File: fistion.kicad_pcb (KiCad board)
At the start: 2 copper layers, 165 x 92.1 mm, 67 parts, among them J1 Conn_01x07, J2 Conn_01x07, J3 Conn_01x04, U1 nice_nano, U2 MT25QL128ABA1ESE

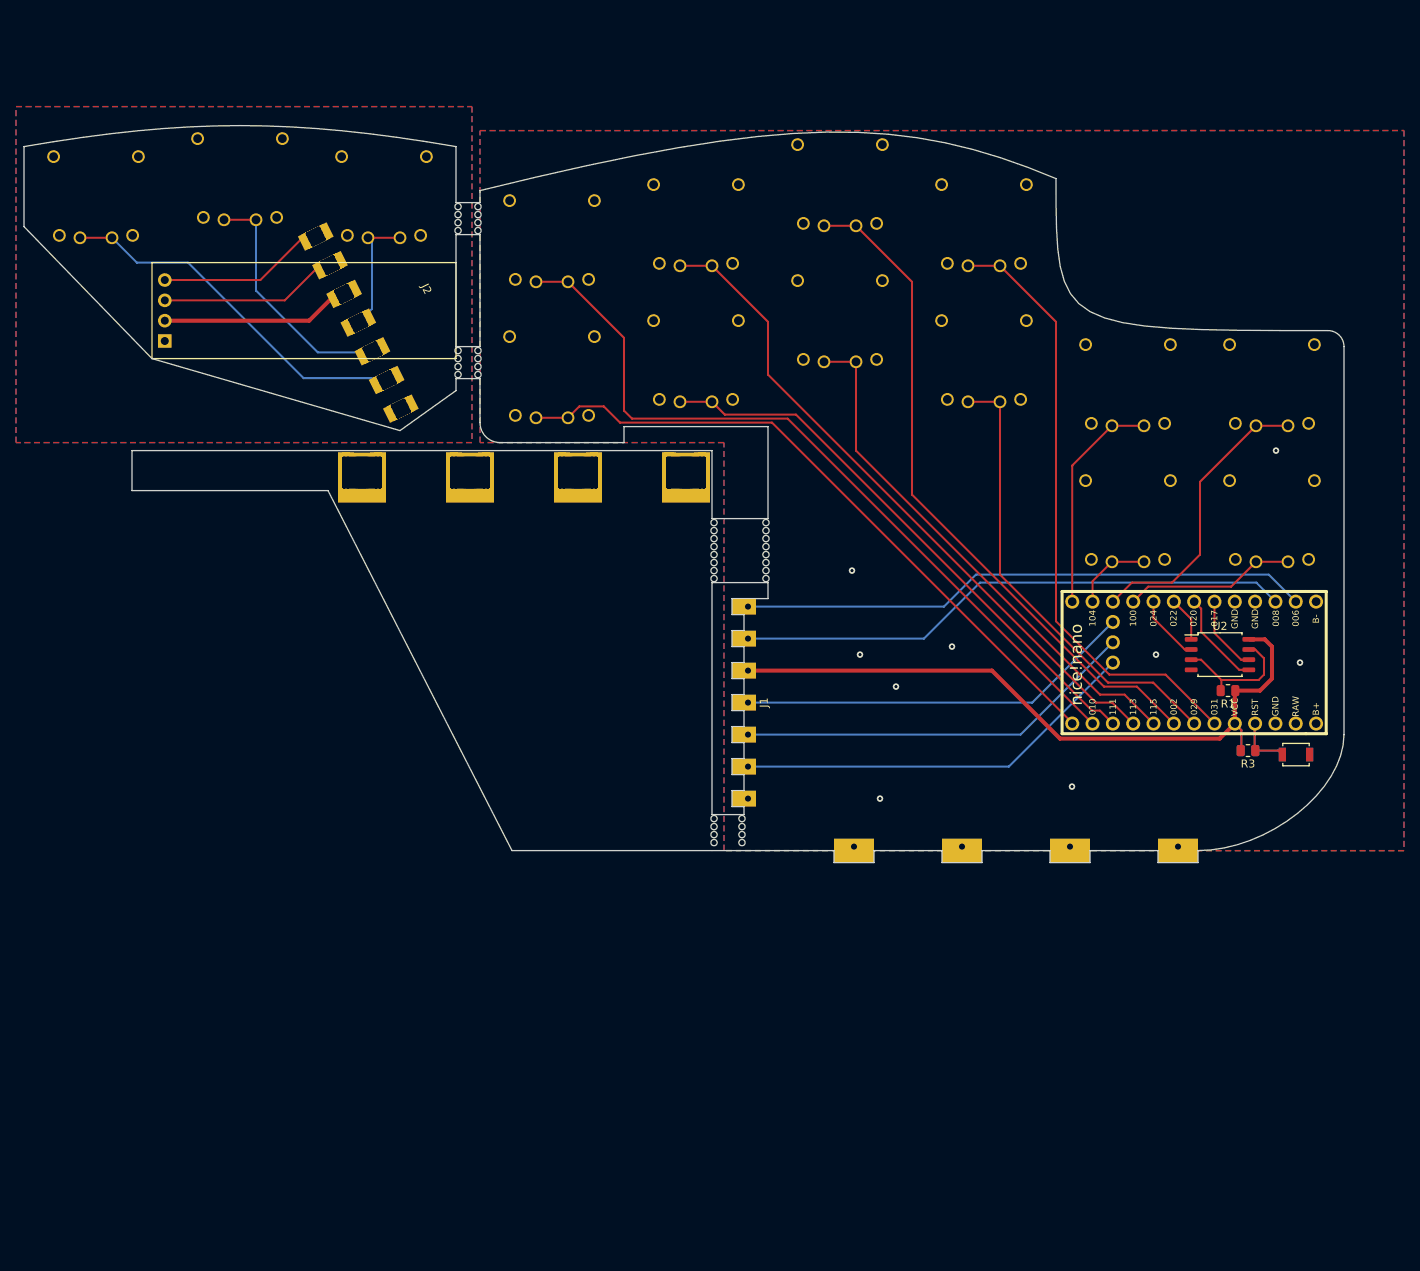
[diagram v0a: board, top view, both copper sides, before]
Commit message: Pending
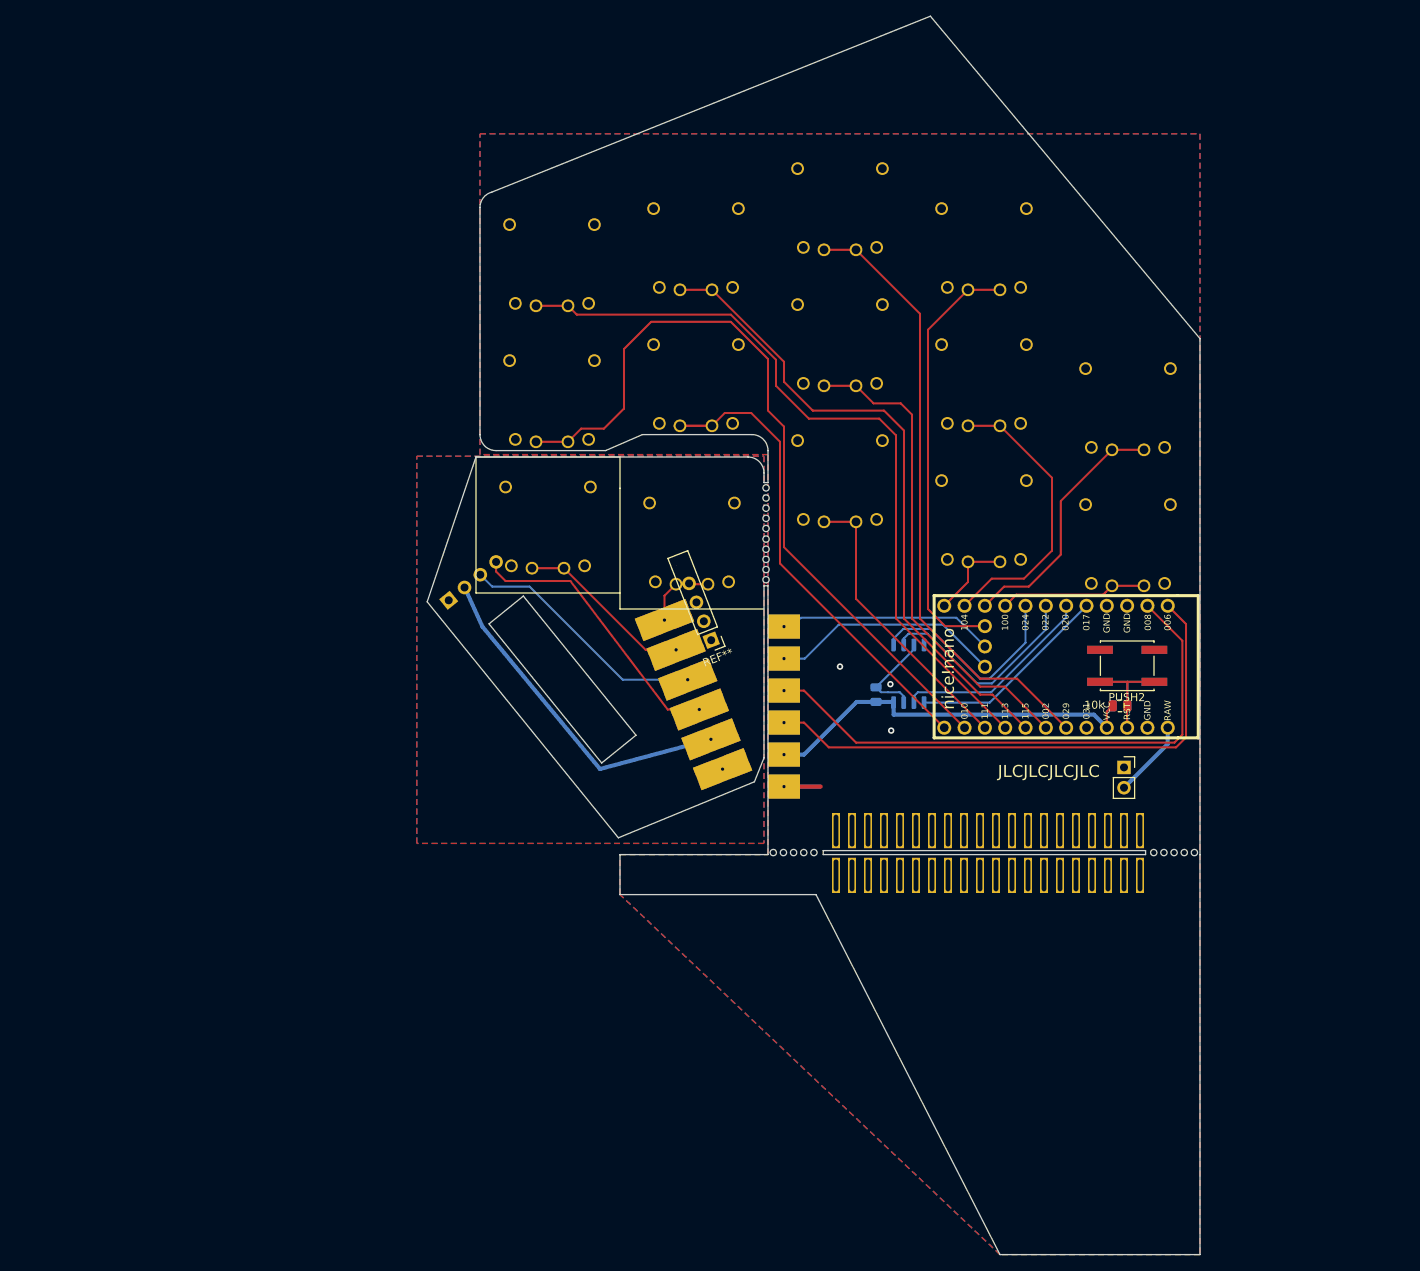
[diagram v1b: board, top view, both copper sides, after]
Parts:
- removed KEY15: SW_Push, lib:Kailh_PG1232
- removed the KEY6 at (169.0, 52.0)
- removed the REF** at (106.0, 71.5)
- removed the REF** at (99.0, 75.5)
- removed the REF** at (99.0, 73.5)
- removed the REF** at (99.0, 76.5)
- removed the REF** at (99.0, 70.5)
- removed the REF** at (99.0, 71.5)
- removed the REF** at (99.0, 69.5)
- removed the REF** at (99.0, 72.5)
- removed the REF** at (103.0, 108.5)
- removed the REF** at (103.0, 107.5)
- removed the REF** at (103.0, 109.5)
- removed the REF** at (106.0, 70.5)
- removed the REF** at (103.0, 106.5)
- removed the REF** at (99.0, 107.5)
- removed the REF** at (99.0, 108.5)
- removed the REF** at (99.0, 106.5)
- removed the REF** at (99.0, 109.5)
- removed the REF** at (70.0, 32.0)
- removed the REF** at (70.0, 31.0)
- removed the REF** at (70.0, 33.0)
- removed the REF** at (70.0, 30.0)
- removed the REF** at (67.0, 31.0)
- removed the REF** at (106.0, 72.5)
- removed the REF** at (67.0, 32.0)
- removed the REF** at (67.0, 30.0)
- removed the REF** at (67.0, 33.0)
- removed the REF** at (70.0, 50.0)
- removed the REF** at (70.0, 49.0)
- removed the REF** at (70.0, 51.0)
- removed the REF** at (70.0, 48.0)
- removed the REF** at (67.0, 49.0)
- removed the REF** at (67.0, 50.0)
- removed the REF** at (67.0, 48.0)
- removed the REF** at (106.0, 69.5)
- removed the REF** at (67.0, 51.0)
- removed the REF** at (106.0, 75.5)
- removed the REF** at (106.0, 74.5)
- removed the REF** at (106.0, 76.5)
- removed the REF** at (106.0, 73.5)
- removed the REF** at (99.0, 74.5)
- removed palm1: Conn_01x04, fistion:palm-female
- removed palm2: Conn_01x04, fistion:palm-male
- added J4: Conn_01x02, Connector_PinSocket_2.54mm:PinSocket_1x02_P2.54mm_Vertical, F.Cu at (150.5, 100.1)
- added KEY11: SW_Push, lib:Kailh_PG1232, F.Cu at (115.0, 64.0)
- added REF**: PinHeader_1x05_P2.54mm_Vertical, Connector_PinHeader_2.54mm:PinHeader_1x05_P2.54mm_Vertical, F.Cu at (98.9, 84.2)
- added REF**: breakaway-mousebites, Keebio-Parts:breakaway-mousebites, F.Cu at (105.5, 74.1)
- added REF**: breakaway-mousebites, Keebio-Parts:breakaway-mousebites, F.Cu at (105.5, 67.7)
- added REF**: breakaway-mousebites, Keebio-Parts:breakaway-mousebites, F.Cu at (109.2, 111.0)
- added REF**: breakaway-mousebites, Keebio-Parts:breakaway-mousebites, F.Cu at (156.8, 111.0)
- added REF**: palm-conn, fistion:palm-conn, F.Cu at (133.5, 113.6)
- added REF**: palm-conn, fistion:palm-conn, F.Cu at (133.5, 108.0)
- J1: value Conn_01x07 -> Conn_01x04; footprint fistion:thumb-male -> steno:OLED
- J2: value Conn_01x07 -> Conn_01x06; footprint fistion:thumb-female -> fistion:thumb-thumb
- J3: value Conn_01x04 -> Conn_01x06; footprint steno:OLED -> fistion:thumb-palm
- PUSH1: renamed from PUSH2; footprint Button_Switch_SMD:SW_SPST_B3U-1000P -> Button_Switch_SMD:SW_SPST_EVQQ2
- PUSH2: renamed from PUSH1; footprint Button_Switch_SMD:SW_SPST_B3U-1000P -> Button_Switch_SMD:SW_SPST_EVQQ2
- R3: renamed from R1; moved to B.Cu
- U2: moved to B.Cu
- moved J3 96.5 mm to (108.0, 92.5), turned to 90 degrees
- moved KEY14 72.6 mm to (96.5, 71.8)
- moved KEY13 70.0 mm to (78.5, 69.8)
- moved J2 62.6 mm to (96.7, 91.0), turned to 111.3 degrees
- moved R3 44.0 mm to (119.5, 91.0), turned to 90 degrees
- moved U2 39.0 mm to (123.6, 88.4), turned to 270 degrees
- moved J1 36.4 mm to (72.7, 71.8), turned to 309 degrees
- moved KEY12 36.0 mm to (133.0, 69.0)
- moved PUSH1 23.8 mm to (150.9, 87.4)
- moved PUSH2 23.8 mm to (150.9, 87.4), turned to 180 degrees
- moved R1 17.0 mm to (150.0, 92.4)
- moved R2 17.0 mm to (150.0, 92.4)
- moved U1 16.0 mm to (142.0, 87.5)
- moved KEY1 3.00 mm to (79.0, 37.0)
- moved KEY10 3.00 mm to (151.0, 72.0)
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- renumbered KEY11 to KEY10, KEY7 to KEY6, KEY8 to KEY7, KEY9 to KEY8, KEY10 to KEY9, R2 to R1, R3 to R2
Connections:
- J1 pad 1: GND -> thumb_gnd
- J1 pad 2: R3C1 -> thumb_vcc
- J1 pad 3: R3C2 -> thumb_scl
- J1 pad 4: R3C3 -> thumb_sda
- J2 pad 2: thumb_R3C1 -> thumb_vcc
- J2 pad 3: thumb_R3C2 -> thumb_sda
- J2 pad 4: thumb_R3C3 -> thumb_scl
- J2 pad 5: thumb_vcc -> thumb_R3C1
- J2 pad 6: thumb_scl -> thumb_R3C2
- J3 pad 1: thumb_gnd -> GND
- J3 pad 2: thumb_vcc -> 3V3
- J3 pad 3: thumb_scl -> SDA
- J3 pad 4: thumb_sda -> SCL
- KEY12 pad 2: R2C6 -> R3C4
- U1 pad 10: R1C6 -> R1C5
- U1 pad 11: R2C5 -> R2C4
- U1 pad 12: R1C5 -> R3C4
- U1 pad 13: R2C1 -> R2C2
- U1 pad 14: R1C1 -> R2C1
- U1 pad 15: R2C2 -> R3C3
- U1 pad 16: R1C2 -> R1C1
- U1 pad 17: R2C3 -> R1C2
- U1 pad 18: R1C3 -> R2C3
- U1 pad 19: R2C4 -> R1C3
- U1 pad 20: R1C4 -> Net-(U1-Pad20)
- U1 pad 24: Net-(U1-Pad24) -> BAT
- U1 pad 31: R3C3 -> R1C4
- U1 pad 5: SCLK -> MOSI
- U1 pad 6: MOSI -> SCLK
- U1 pad 7: CS -> MISO
- U1 pad 8: MISO -> CS
- U1 pad 9: R2C6 -> R2C5
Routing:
- net 3V3: track 89.3 -> 51.3 mm
- net R1C6: track 36.3 -> 0.00 mm
- net R3C2: track 50.4 -> 26.0 mm
- net thumb_R3C1: track 45.7 -> 22.2 mm
- net R3C1: track 51.0 -> 28.0 mm
- net R1C4: track 76.4 -> 54.0 mm
- net thumb_R3C2: track 30.7 -> 9.08 mm
- net R2C4: track 57.6 -> 36.1 mm
- net R2C6: track 21.4 -> 0.00 mm
- net CS: track 5.61 -> 26.8 mm
- net thumb_vcc: track 23.8 -> 42.8 mm
- net MISO: track 8.40 -> 27.2 mm
- net SCLK: track 9.60 -> 25.4 mm
- net thumb_R3C3: track 15.5 -> 0.00 mm
- net thumb_sda: track 21.1 -> 35.1 mm
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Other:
- board size 165 x 92.1 mm -> 96.6 x 154.8 mm
